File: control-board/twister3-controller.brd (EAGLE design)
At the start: 191 x 90.5 mm, 61 parts, among them J2 OSTVN04A150, J7 BARREL-JACK_PJ-063BH, U1 MAX6816, U10 Teensy 3.2, U11 TMC2130-LA, U2 GDM1602K, U3 IS31FL3193, U4 MIC4680-5.0YM-TR

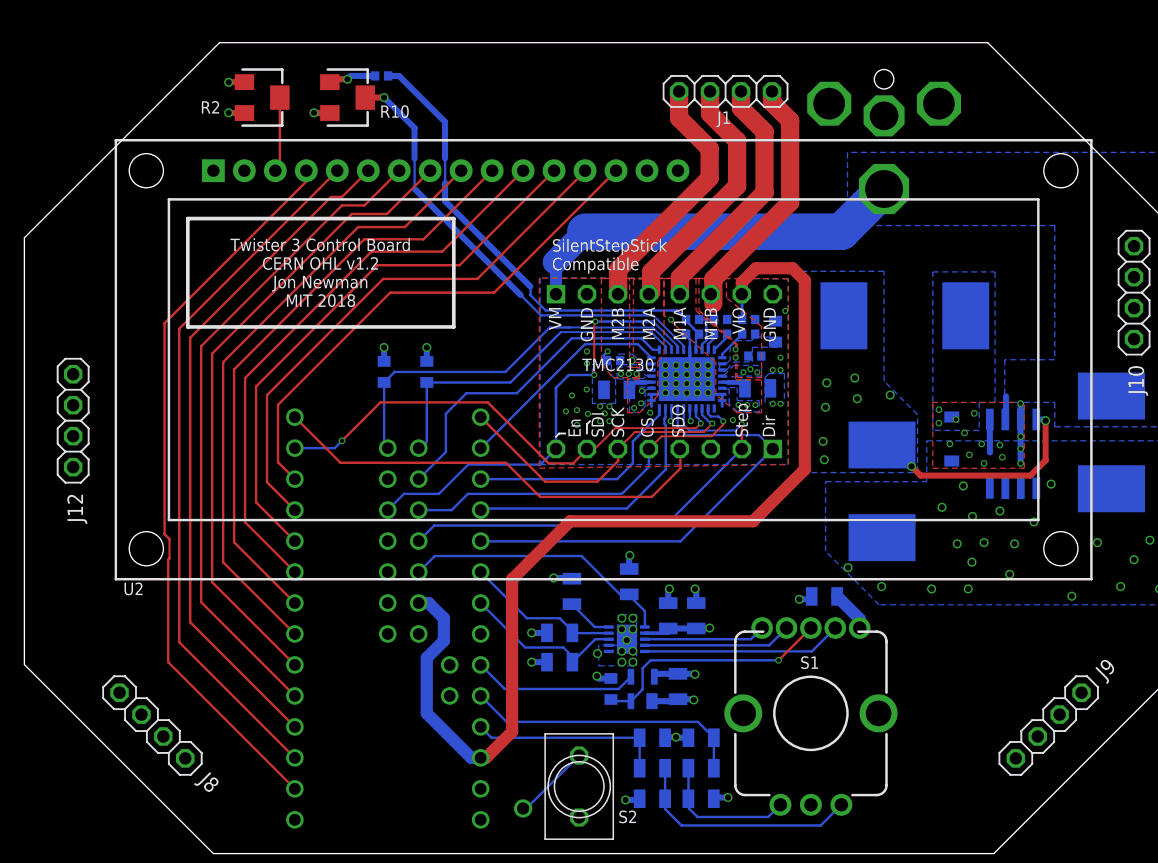
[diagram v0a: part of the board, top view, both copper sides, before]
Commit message: Complete rev 1.0 of control board
- Off to fab
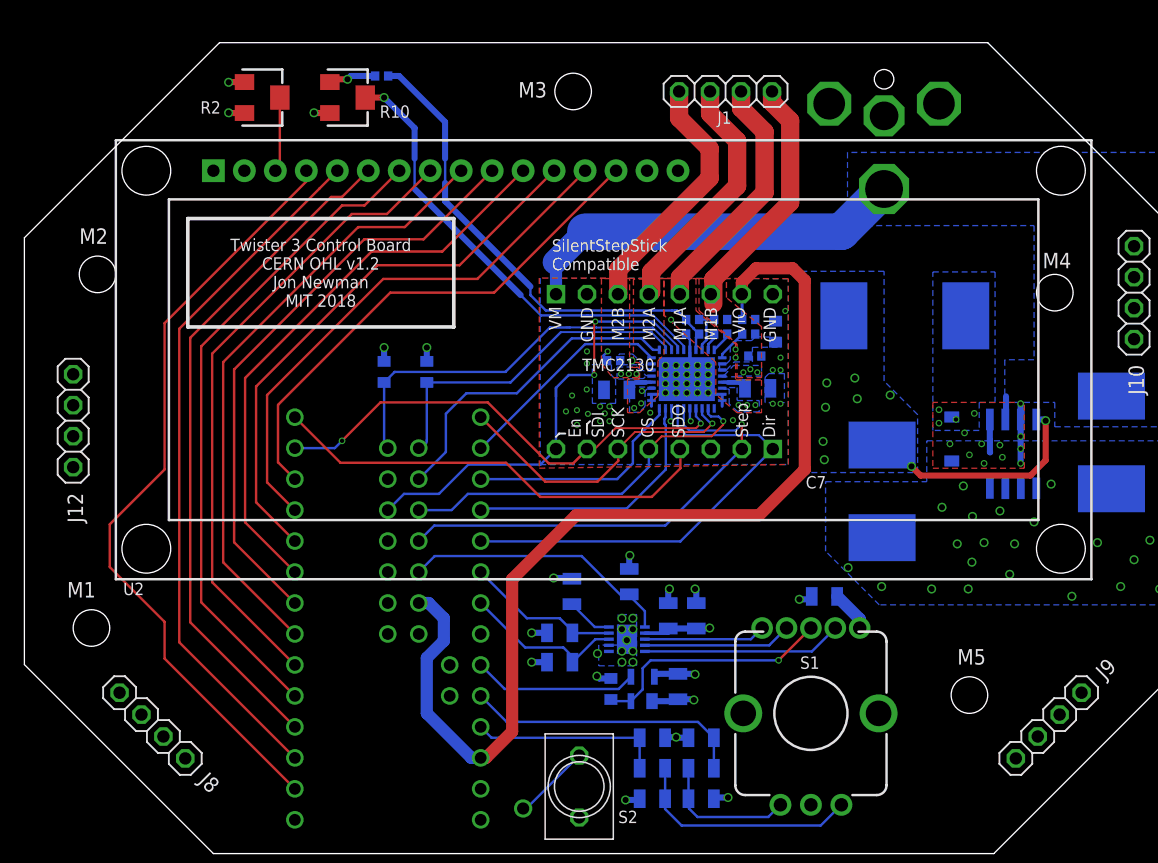
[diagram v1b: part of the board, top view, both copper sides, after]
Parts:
- U2: device SparkFun-Displays:LCD-16X2 -> jonnew:LCD-16X2
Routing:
- net RS: track 60.0 -> 63.7 mm
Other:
- board text added: "- Board to panel stack height: 12 mm. - Teensy goes on bottom with top of teensy facing up (when board is flipped) - Silent stepper stick goes on bottom with top of module facing down (whe board flipped)"
- board text added: "M1"
- board text added: "M2"
- board text added: "M3"
- board text added: "M4"
- board text added: "M5"
- board text removed: "- Teensy goes on bottom with top of board facing up. - Silent stepper stick goes on bottom with top of board facing down - Inner holes are for 1/2" standoffs"
- board text removed: "0.5" standoffs"
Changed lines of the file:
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@@
 <setting verticaltext="up"/>
 </settings>
-<grid distance="0.001429" unitdist="inch" unit="inch" style="lines" multiple="1" display="yes" altdistance="5" altunitdist="mil" altunit="mil"/>
+<grid distance="0.5" unitdist="mm" unit="mm" style="lines" multiple="1" display="yes" altdistance="5" altunitdist="mil" altunit="mil"/>
 <layers>
 <layer number="1" name="Top" color="4" fill="1" visible="yes" active="yes"/>
@@
 <layer number="37" name="tTest" color="7" fill="1" visible="no" active="yes"/>
 <layer number="38" name="bTest" color="7" fill="1" visible="no" active="yes"/>
-<layer number="39" name="tKeepout" color="4" fill="11" visible="no" active="yes"/>
+<layer number="39" name="tKeepout" color="4" fill="11" visible="yes" active="yes"/>
 <layer number="40" name="bKeepout" color="1" fill="11" visible="no" active="yes"/>
 <layer number="41" name="tRestrict" color="4" fill="10" visible="no" active="yes"/>
 <layer number="42" name="bRestrict" color="1" fill="10" visible="no" active="yes"/>
 <layer number="43" name="vRestrict" color="2" fill="10" visible="no" active="yes"/>
-<layer number="44" name="Drills" color="7" fill="1" visible="no" active="yes"/>
-<layer number="45" name="Holes" color="7" fill="1" visible="no" active="yes"/>
+<layer number="44" name="Drills" color="7" fill="1" visible="yes" active="yes"/>
+<layer number="45" name="Holes" color="7" fill="1" visible="yes" active="yes"/>
 <layer number="46" name="Milling" color="3" fill="1" visible="no" active="yes"/>
 <layer number="47" name="Measures" color="7" fill="1" visible="no" active="yes"/>
@@
 <layer number="49" name="Reference" color="7" fill="1" visible="no" active="yes"/>
 <layer number="50" name="dxf" color="7" fill="1" visible="no" active="no"/>
-<layer number="51" name="tDocu" color="7" fill="1" visible="no" active="yes"/>
+<layer number="51" name="tDocu" color="7" fill="1" visible="yes" active="yes"/>
 <layer number="52" name="bDocu" color="7" fill="1" visible="no" active="yes"/>
 <layer number="53" name="tGND_GNDA" color="7" fill="9" visible="no" active="no"/>
@@
 <hole x="187.8" y="63.39" drill="3"/>
 <hole x="187.8" y="3.85" drill="3"/>
-<text x="-7" y="-4.1" size="1.016" layer="51" rot="R180">0.5" standoffs</text>
 <wire x1="95.5" y1="1" x2="95.5" y2="-1" width="0.127" layer="51"/>
 <wire x1="94.5" y1="0" x2="96.5" y2="0" width="0.127" layer="51"/>
-<text x="95.5" y="-3" size="1.016" layer="51">Top Board Origin</text>
+<text x="96.5" y="-2" size="1.016" layer="51">Top Board Origin</text>
 <wire x1="0.5" y1="51" x2="0.5" y2="16" width="0" layer="20"/>
 <wire x1="0.5" y1="16" x2="16" y2="0.5" width="0" layer="20"/>
@@
 <wire x1="108.5" y1="27.5" x2="178.5" y2="27.5" width="0" layer="20"/>
 <wire x1="179.5" y1="28.5" x2="179.5" y2="53.5" width="0" layer="20"/>
-<text x="18.1" y="-23.2" size="1.016" layer="51">- Teensy goes on bottom with top of board facing up.
-- Silent stepper stick goes on bottom with top of board facing down
-- Inner holes are for 1/2" standoffs</text>
 <circle x="160.5" y="12" radius="4.75" width="0.05" layer="20"/>
 <wire x1="178.5" y1="54.5" x2="108.5" y2="54.5" width="0" layer="20"/>
-<wire x1="-6.5" y1="-4" x2="10" y2="10.4" width="0.01" layer="51"/>
 <wire x1="107.5" y1="53.5" x2="108.5" y2="54.5" width="0" layer="20" curve="-233.130102"/>
 <wire x1="108.5" y1="27.5" x2="107.5" y2="28.5" width="0" layer="20" curve="-233.130102"/>
@@
 <rectangle x1="127.2643875" y1="60.579" x2="127.59204375" y2="60.61506875" layer="21"/>
 <rectangle x1="113.728728125" y1="60.61506875" x2="113.982728125" y2="60.6513875" layer="21"/>
+<hole x="85" y="46.5" drill="3"/>
+<hole x="6.5" y="48" drill="3"/>
+<hole x="6" y="19" drill="3"/>
+<circle x="85" y="46.5" radius="3.5" width="0" layer="39"/>
+<circle x="6.5" y="48" radius="3.5" width="0" layer="39"/>
+<circle x="6" y="19" radius="3.5" width="0" layer="39"/>
+<circle x="78" y="13.5" radius="3.5" width="0" layer="39"/>
+<hole x="78" y="13.5" drill="3"/>
+<circle x="45.5" y="63" radius="3.5" width="0" layer="39"/>
+<hole x="45.5" y="63" drill="3"/>
+<text x="4" y="21.5" size="1.27" layer="21" font="vector" ratio="18">M1</text>
+<text x="5" y="50.5" size="1.27" layer="21" font="vector" ratio="18">M2</text>
+<text x="41" y="62.5" size="1.27" layer="21" font="vector" ratio="18">M3</text>
+<text x="84" y="48.5" size="1.27" layer="21" font="vector" ratio="18">M4</text>
+<text x="77" y="16" size="1.27" layer="21" font="vector" ratio="18">M5</text>
+<text x="17.5" y="77" size="1.27" layer="51" font="vector" ratio="18">- Board to panel stack height:  12 mm.
+- Teensy goes on bottom with top of teensy facing up (when board is flipped)
+- Silent stepper stick goes on bottom with top of module facing down (whe board flipped)</text>
 </plain>
 <attributes>
@@
 <attribute name="VALUE" x="49.54" y="11.25" size="1.016" layer="28" font="vector" ratio="19" rot="MR0"/>
 </element>
-<element name="U2" library="SparkFun-Displays" package="LCD-16X2" value="GDM1602K" x="48" y="41" smashed="yes">
+<element name="U2" library="jonnew" package="LCD-16X2" value="GDM1602K" x="48" y="41" smashed="yes">
 <attribute name="NAME" x="8.6" y="21.7" size="1.016" layer="25" font="vector" ratio="19"/>
 <attribute name="SF_ID" value="LCD-00255" x="48" y="41" size="1.778" layer="27" display="off"/>
@@
 <attribute name="DK" value="" x="55.6" y="20" size="1.778" layer="28" rot="MR90" display="off"/>
 <attribute name="MN" value="TDK Corp." x="55.6" y="20" size="1.778" layer="28" rot="MR90" display="off"/>
-<attribute name="NAME" x="57.04" y="22.75" size="1.016" layer="26" font="vector" ratio="19" rot="MR90"/>
+<attribute name="NAME" x="58.54" y="19.75" size="1.016" layer="26" font="vector" ratio="19" rot="MR90"/>
 <attribute name="PARTNO" value="C2012X5R1Cxxxxxxx" x="55.6" y="20" size="1.778" layer="28" rot="MR90" display="off"/>
-<attribute name="VALUE" x="55.79" y="22.75" size="1.016" layer="28" font="vector" ratio="19" rot="MR90"/>
+<attribute name="VALUE" x="57.29" y="19.75" size="1.016" layer="28" font="vector" ratio="19" rot="MR90"/>
 <attribute name="VID" value="DK" x="55.6" y="20" size="1.778" layer="28" rot="MR90" display="off"/>
 </element>
@@
 </element>
 <element name="C7" library="jonnew" package="7343M" value="T491D227M010AT" x="70.838" y="30.206" smashed="yes" rot="MR270">
-<attribute name="NAME" x="65.54" y="23.75" size="1.016" layer="26" font="vector" ratio="19" rot="MR90"/>
-<attribute name="VALUE" x="64.29" y="23.75" size="1.016" layer="28" font="vector" ratio="19" rot="MR90"/>
+<attribute name="NAME" x="66.25" y="31.46" size="1.016" layer="25" font="vector" ratio="19" rot="R180"/>
+<attribute name="VALUE" x="66.25" y="30.21" size="1.016" layer="27" font="vector" ratio="19" rot="R180"/>
 </element>
 <element name="C8" library="jonnew" package="7343M" value="T491D156K035AT" x="89.648" y="34.22" smashed="yes" rot="MR270">
@@
 <wire x1="38.35" y1="8.35" x2="40.5" y2="10.5" width="1" layer="1"/>
 <wire x1="40.5" y1="10.5" x2="40.5" y2="23" width="1" layer="1"/>
-<wire x1="40.5" y1="23" x2="45.25" y2="27.75" width="1" layer="1"/>
-<wire x1="45.25" y1="27.75" x2="60.25" y2="27.75" width="1" layer="1"/>
-<wire x1="60.25" y1="27.75" x2="64.5" y2="32" width="1" layer="1"/>
+<wire x1="60.75" y1="28.25" x2="64.5" y2="32" width="1" layer="1"/>
 <wire x1="60.5" y1="48.5" x2="63.5" y2="48.5" width="1" layer="1"/>
 <wire x1="63.5" y1="48.5" x2="64.5" y2="47.5" width="1" layer="1"/>
@@
 <wire x1="34.9" y1="19.8" x2="34.9" y2="17.95" width="1" layer="16"/>
 <wire x1="34.9" y1="17.95" x2="33.5" y2="16.55" width="1" layer="16"/>
+<wire x1="45.75" y1="28.25" x2="60.75" y2="28.25" width="1" layer="1"/>
+<wire x1="40.5" y1="23" x2="45.75" y2="28.25" width="1" layer="1"/>
 </signal>
 <signal name="N$4">
@@
 <contactref element="U2" pad="4"/>
 <contactref element="U10" pad="0"/>
-<wire x1="12.4" y1="24.71299375" x2="12.4" y2="26.28700625" width="0.2" layer="1"/>
-<wire x1="12.4" y1="26.28700625" x2="12" y2="26.68700625" width="0.2" layer="1"/>
-<wire x1="12.3" y1="24.61299375" x2="12.4" y2="24.71299375" width="0.2" layer="1"/>
-<wire x1="12.3" y1="16.19" x2="12.3" y2="24.61299375" width="0.2" layer="1"/>
 <wire x1="23.62" y1="55.62" x2="12" y2="44" width="0.2" layer="1"/>
-<wire x1="12" y1="26.68700625" x2="12" y2="44" width="0.2" layer="1"/>
-<wire x1="22.68" y1="5.81" x2="12.3" y2="16.19" width="0.2" layer="1"/>
+<wire x1="12" y1="44" x2="12" y2="32" width="0.2" layer="1"/>
 <wire x1="23.62" y1="56.5" x2="23.62" y2="55.62" width="0.2" layer="1"/>
+<wire x1="12" y1="19.5" x2="12" y2="16.49" width="0.2" layer="1"/>
+<wire x1="12" y1="16.49" x2="22.68" y2="5.81" width="0.2" layer="1"/>
+<wire x1="12" y1="32" x2="7.5" y2="27.5" width="0.2" layer="1"/>
+<wire x1="7.5" y1="27.5" x2="7.5" y2="24" width="0.2" layer="1"/>
+<wire x1="7.5" y1="24" x2="12" y2="19.5" width="0.2" layer="1"/>
 </signal>
 <signal name="RW">
@@
 <vertex x="68" y="58"/>
 <vertex x="68" y="52"/>
-<vertex x="85" y="52"/>
-<vertex x="85" y="41"/>
+<vertex x="83.3" y="52"/>
+<vertex x="83.3" y="41"/>
 <vertex x="80.9" y="41"/>
 <vertex x="80.9" y="37.5"/>
